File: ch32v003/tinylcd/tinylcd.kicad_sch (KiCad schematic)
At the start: 16 parts, among them J1 APPLE, J2 USB_C_Receptacle_USB2.0, J3 PGM, J4 Micro_SD_Card_Det1, U1 RB017A1505A_Connector, U3 CH32V003F4U6, U4 3.3vReg

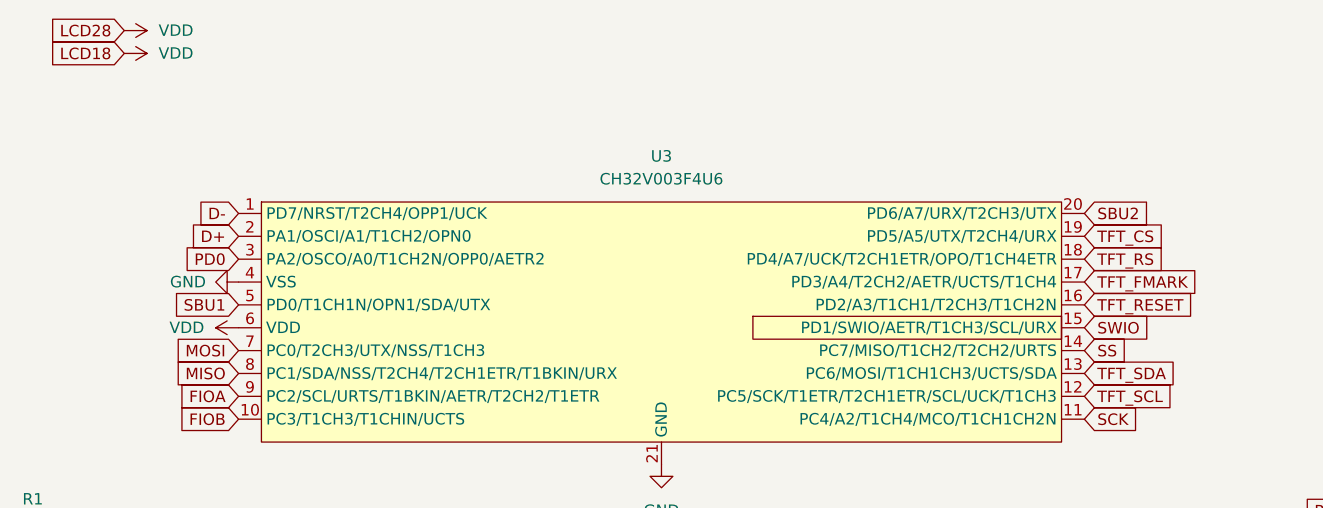
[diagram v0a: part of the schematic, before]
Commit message: Oops a few fixes.
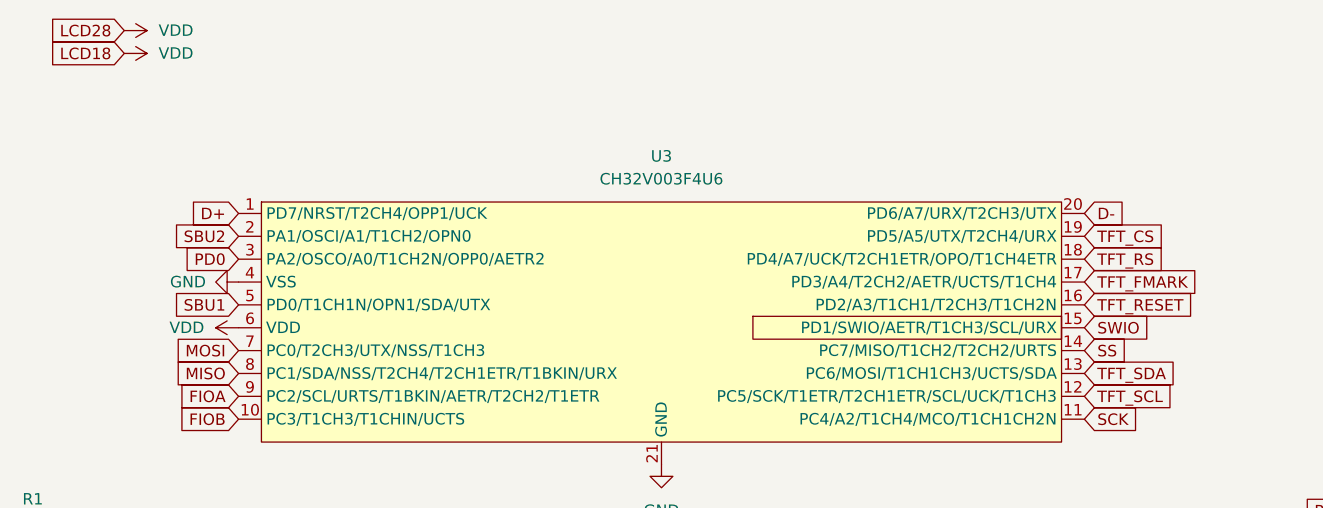
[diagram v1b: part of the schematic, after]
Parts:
- J3: LCSC (none) -> NP
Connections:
- net D+: now also U3.1 (PD7/NRST/T2CH4/OPP1/UCK); no longer U3.2 (PA1/OSCI/A1/T1CH2/OPN0)
- net D-: now also U3.20 (PD6/A7/URX/T2CH3/UTX); no longer U3.1 (PD7/NRST/T2CH4/OPP1/UCK)
- net SBU2: now also U3.2 (PA1/OSCI/A1/T1CH2/OPN0); no longer U3.20 (PD6/A7/URX/T2CH3/UTX)
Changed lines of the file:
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@@
-    )
-  )
-  (global_label "D-" (shape input) (at 97.79 52.07 180) (fields_autoplaced)
-    (effects (font (size 1.27 1.27)) (justify right))
-    (property "Intersheetrefs" "${INTERSHEET_REFS}" (at 92.5345 51.9906 0)
-      (effects (font (size 1.27 1.27)) (justify right) hide)
     )
   )
@@
     )
   )
+  (global_label "SBU2" (shape input) (at 97.79 54.61 180) (fields_autoplaced)
+    (effects (font (size 1.27 1.27)) (justify right))
+    (property "Intersheetrefs" "${INTERSHEET_REFS}" (at 89.7853 54.61 0)
+      (effects (font (size 1.27 1.27)) (justify right) hide)
+    )
+  )
   (global_label "SCK" (shape input) (at 66.04 123.19 0) (fields_autoplaced)
     (effects (font (size 1.27 1.27)) (justify left))
@@
     )
   )
+  (global_label "D+" (shape input) (at 97.79 52.07 180) (fields_autoplaced)
+    (effects (font (size 1.27 1.27)) (justify right))
+    (property "Intersheetrefs" "${INTERSHEET_REFS}" (at 91.9624 52.07 0)
+      (effects (font (size 1.27 1.27)) (justify right) hide)
+    )
+  )
   (global_label "TFT_LEDA" (shape input) (at 41.91 74.93 180) (fields_autoplaced)
     (effects (font (size 1.27 1.27)) (justify right))
@@
     )
   )
-  (global_label "D+" (shape input) (at 97.79 54.61 180) (fields_autoplaced)
-    (effects (font (size 1.27 1.27)) (justify right))
-    (property "Intersheetrefs" "${INTERSHEET_REFS}" (at 92.5345 54.5306 0)
-      (effects (font (size 1.27 1.27)) (justify right) hide)
-    )
-  )
   (global_label "LCD28" (shape input) (at 60.96 57.15 0) (fields_autoplaced)
     (effects (font (size 1.27 1.27)) (justify left))
@@
     )
   )
-  (global_label "SBU2" (shape input) (at 191.77 52.07 0) (fields_autoplaced)
-    (effects (font (size 1.27 1.27)) (justify left))
-    (property "Intersheetrefs" "${INTERSHEET_REFS}" (at 199.2026 51.9906 0)
-      (effects (font (size 1.27 1.27)) (justify left) hide)
-    )
-  )
   (global_label "TFT_CS" (shape input) (at 41.91 54.61 180) (fields_autoplaced)
     (effects (font (size 1.27 1.27)) (justify right))
@@
     (property "Intersheetrefs" "${INTERSHEET_REFS}" (at 29.7602 64.6906 0)
       (effects (font (size 1.27 1.27)) (justify right) hide)
+    )
+  )
+  (global_label "D-" (shape input) (at 191.77 52.07 0) (fields_autoplaced)
+    (effects (font (size 1.27 1.27)) (justify left))
+    (property "Intersheetrefs" "${INTERSHEET_REFS}" (at 197.5976 52.07 0)
+      (effects (font (size 1.27 1.27)) (justify left) hide)
     )
   )
@@
       (effects (font (size 1.27 1.27)) hide)
     )
+    (property "LCSC" "NP" (at 236.22 67.31 0)
+      (effects (font (size 1.27 1.27)) hide)
+    )
